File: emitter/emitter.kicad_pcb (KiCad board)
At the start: 2 copper layers, 31.4 x 26.4 mm, 17 parts, among them J1 1935174

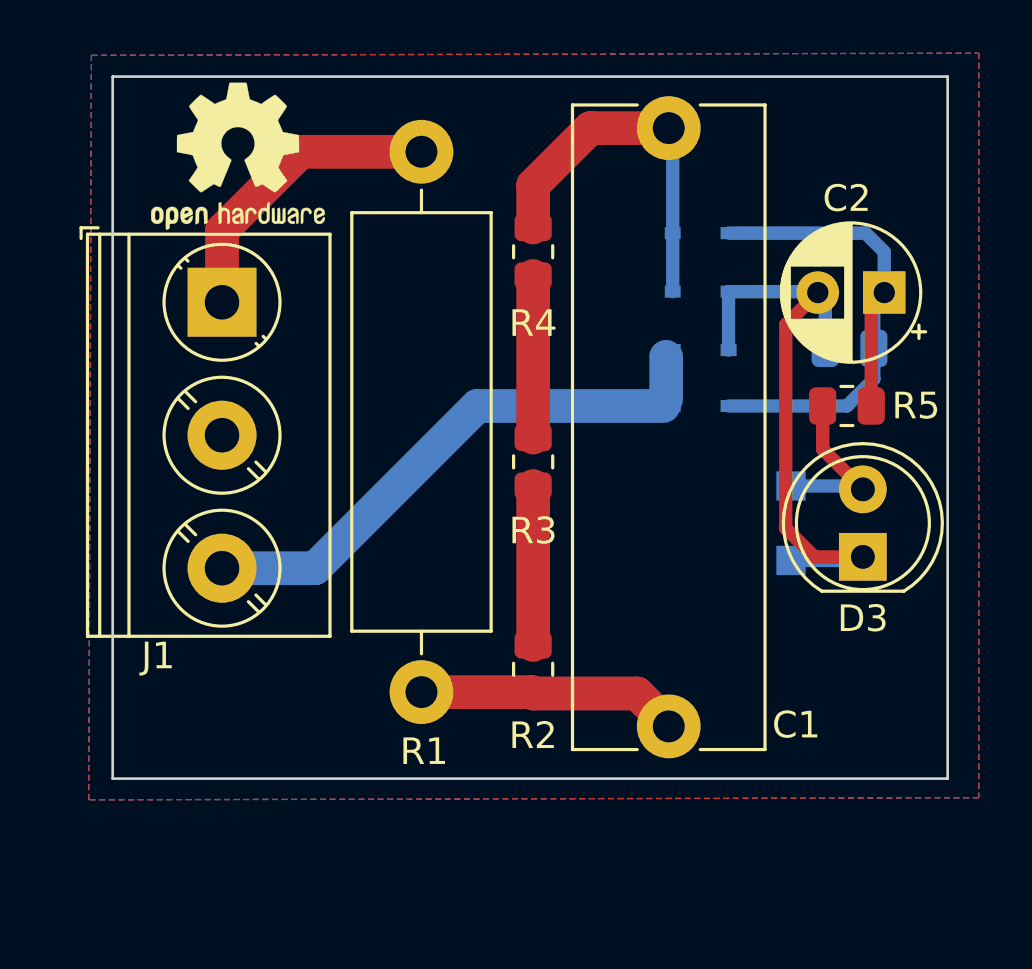
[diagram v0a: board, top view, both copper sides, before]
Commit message: Updated rev
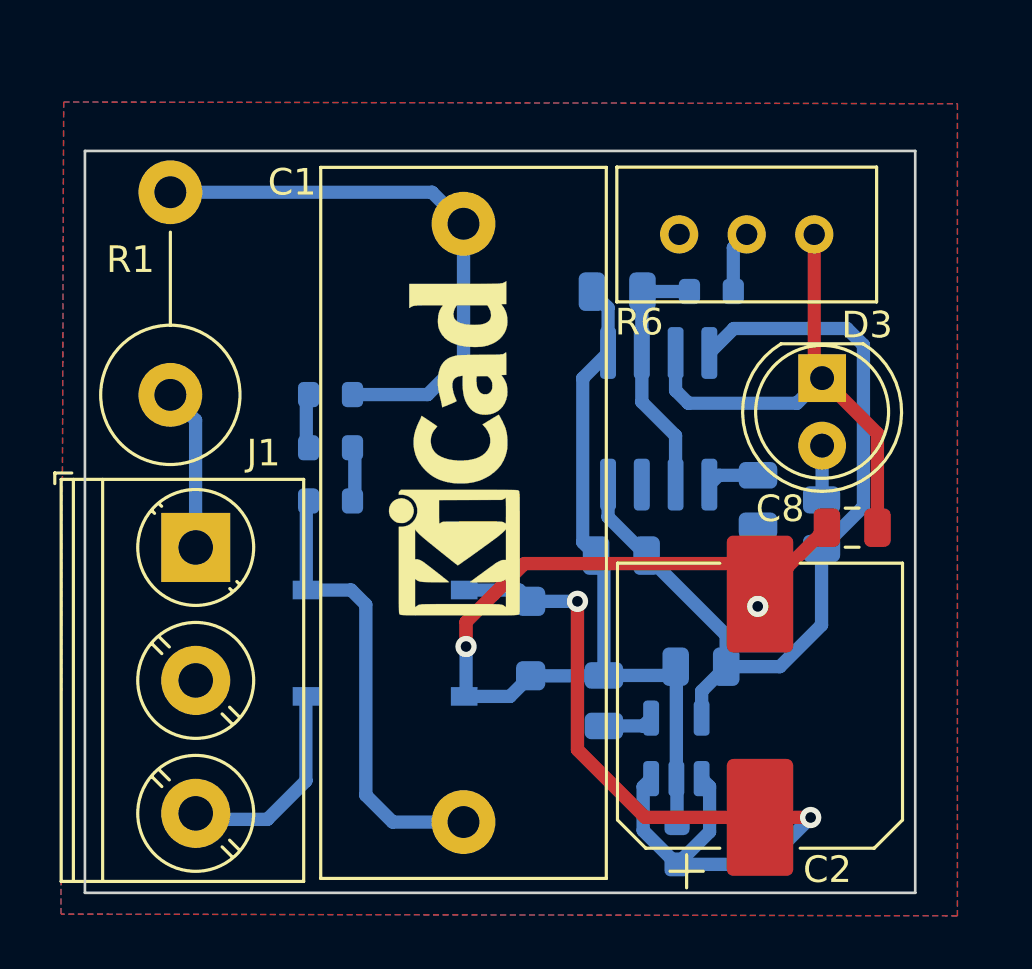
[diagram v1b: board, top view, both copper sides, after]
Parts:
- removed D2, D5, D6: 1N4148WS, Diode_SMD:D_SOD-323
- removed D4: 5V1, Diode_SMD:D_SOD-123F
- added C3: 10nF, Capacitor_SMD:C_0805_2012Metric, B.Cu at (84.9, 36.4)
- added C4: 1nF, Capacitor_SMD:C_0805_2012Metric, B.Cu at (84.8, 26.5)
- added C5: 1u, Capacitor_SMD:C_0603_1608Metric, B.Cu at (87.0, 47.3)
- added C6: 10nF, Capacitor_SMD:C_0805_2012Metric, B.Cu at (84.3, 41.9)
- added C7: 2.2uF, Capacitor_SMD:C_0805_2012Metric, B.Cu at (87.9, 40.6)
- added C8: 10nF, Capacitor_SMD:C_0805_2012Metric, F.Cu at (93.6, 35.4)
- added C9: 100nF, Capacitor_SMD:C_0805_2012Metric, B.Cu at (90.1, 34.4)
- added D7: ABS6, Diode_SMD:Diode_Bridge_Diotec_ABS, B.Cu at (76.0, 39.7)
- added R7: 15k, Resistor_SMD:R_0603_1608Metric, B.Cu at (88.3, 26.5)
- added U1: TLC555xD, Package_SO:SOIC-8_3.9x4.9mm_P1.27mm, B.Cu at (86.3, 31.3)
- added U2: LP2985-5.0, Package_TO_SOT_SMD:SOT-23-5, B.Cu at (87.0, 43.7)
- C1: value 330n -> 1u; footprint Capacitor_THT:C_Rect_L24.0mm_W7.0mm_P22.50mm_MKT -> Capacitor_THT:C_Rect_L26.5mm_W10.5mm_P22.50mm_MKS4
- C2: value c=68u -> 68u; footprint Capacitor_THT:CP_Radial_D5.0mm_P2.50mm -> Capacitor_SMD:CP_Elec_10x12.5
- D1: value 1N4148WS -> MM1Z4734A; footprint Diode_SMD:D_SOD-323 -> Diode_SMD:D_SOD-123F
- D3: value IR 5mm 20mA -> IR 5mm 65mA
- R1: value 10 -> 100; footprint Resistor_THT:R_Axial_DIN0516_L15.5mm_D5.0mm_P20.32mm_Horizontal -> Resistor_THT:R_Axial_DIN0516_L15.5mm_D5.0mm_P7.62mm_Vertical
- R2, R3, R4: footprint Resistor_SMD:R_0805_2012Metric -> Resistor_SMD:R_0603_1608Metric; moved to B.Cu
- R5: value 470 -> 60; moved to B.Cu
- R6: value 47k -> 5k; footprint Resistor_SMD:R_0805_2012Metric -> Potentiometer_THT:Potentiometer_Bourns_3296W_Vertical; moved to F.Cu
- REF**: moved to F.Cu
- REF**: moved to B.Cu
- moved C1 20.4 mm to (79.0, 23.9), turned to -90 degrees
- moved D1 16.5 mm to (81.5, 39.5), turned to -90 degrees
- moved C2 16.2 mm to (90.1, 42.1), turned to 90 degrees
- moved R1 13.1 mm to (68.0, 30.4), turned to 90 degrees
- moved R2 12.8 mm to (74.0, 30.4), turned to 180 degrees
- moved R4 12.1 mm to (74.0, 34.4), turned to 180 degrees
- moved J1 9.27 mm to (68.9, 36.1)
- moved R3 7.64 mm to (74.0, 32.4), turned to 0 degrees
- moved D3 6.90 mm to (92.5, 29.8), turned to -90 degrees
- moved REF** 4.91 mm to (73.4, 25.4), turned to 180 degrees
- moved REF** 4.69 mm to (79.2, 32.4), turned to 90 degrees
- moved R5 4.55 mm to (92.4, 35.2), turned to 90 degrees
- moved R6 4.49 mm to (92.2, 24.3), turned to 0 degrees
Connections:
- C1 pad 2: Net-(D1-A) -> Net-(C1-Pad2)
- C2 pad 1: Net-(D1-K) -> +5VA
- C2 pad 2: Net-(D2-A) -> GND
- D1 pad 1: Net-(D1-K) -> +5VA
- D1 pad 2: Net-(D1-A) -> GND
- D3 pad 1: Net-(D2-A) -> Net-(D3-K)
- R4 pad 2: Net-(D1-A) -> Net-(C1-Pad2)
- R5 pad 1: Net-(D1-K) -> +5V
- R6 pad 1: Net-(D1-K) -> Net-(D3-K)
- R6 pad 2: Net-(D2-A) -> Net-(R6-Pad2)
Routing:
- net GND: track 0.00 -> 53.3 mm, vias 0 -> 2
- net +5V: track 0.00 -> 33.4 mm
- net +5VA: track 0.00 -> 33.3 mm, vias 0 -> 2
- net Net-(D2-A): track 23.3 -> 0.00 mm
- net Net-(D1-K): track 21.4 -> 0.00 mm
- net Net-(D3-K): track 0.00 -> 19.5 mm
- net Net-(C1-Pad2): track 0.00 -> 17.1 mm
- net Net-(D1-A): track 13.8 -> 0.00 mm
- net /N: track 20.7 -> 7.93 mm
- net Net-(C1-Pad1): track 9.86 -> 21.2 mm
- net Net-(U1-THR): track 0.00 -> 9.56 mm
- net /L: track 11.4 -> 6.36 mm
- net Net-(D3-A): track 6.51 -> 2.05 mm
- net Net-(R3-Pad2): track 6.07 -> 2.00 mm
- net Net-(R2-Pad2): track 5.98 -> 2.00 mm
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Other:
- board size 31.4 x 26.4 mm -> 31.2 x 27.9 mm
